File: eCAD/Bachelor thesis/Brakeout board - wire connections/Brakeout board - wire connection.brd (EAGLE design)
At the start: 20 x 13.5 mm, 5 parts

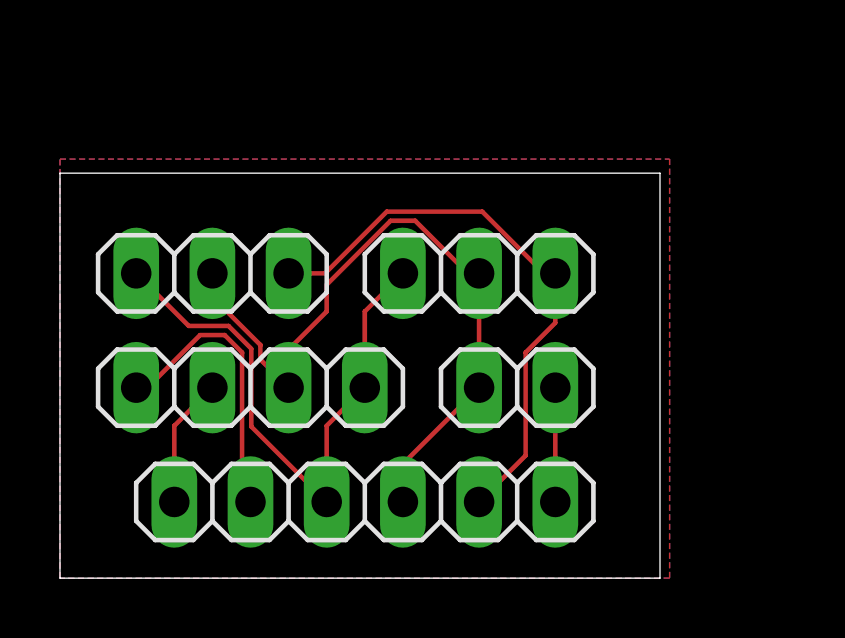
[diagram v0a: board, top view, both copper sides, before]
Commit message: Final touches
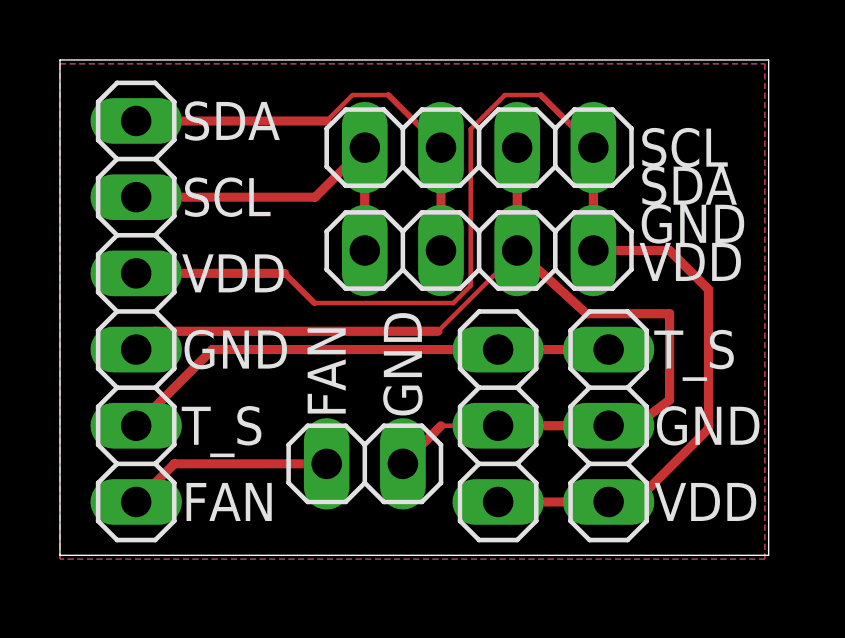
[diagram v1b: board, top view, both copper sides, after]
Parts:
- added I2C_RES: (no value), pinhead:1X04
- moved DS18B20_1 14.2 mm to (18.3, 5.08), turned to 90 degrees
- moved OUTPUT 9.92 mm to (2.54, 8.89), turned to 90 degrees
- moved VEML7700 8.89 mm to (14.0, 10.9)
- moved FAN 5.68 mm to (10.2, 3.81), turned to 0 degrees
- moved DS18B20_2 5.12 mm to (14.6, 5.08), turned to 90 degrees
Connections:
- net GND: now also I2C_RES.2
- net SCL: now also I2C_RES.4
- net SDA: now also I2C_RES.3
- net SENSE_VDD33: now also I2C_RES.1
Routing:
- net SENSE_VDD33: track 19.7 -> 42.8 mm
- net GND: track 24.6 -> 36.0 mm
- net SDA: track 4.34 -> 14.7 mm
- net VDD_FAN: track 3.81 -> 6.88 mm
- net DS18B_SIG: track 19.3 -> 16.8 mm
- net SCL: track 9.59 -> 11.7 mm
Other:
- board size 20 x 13.5 mm -> 23.6 x 16.5 mm
